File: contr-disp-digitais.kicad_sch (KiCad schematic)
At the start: 25 parts, among them U1 TL081, U2 TL081, U3 TL081

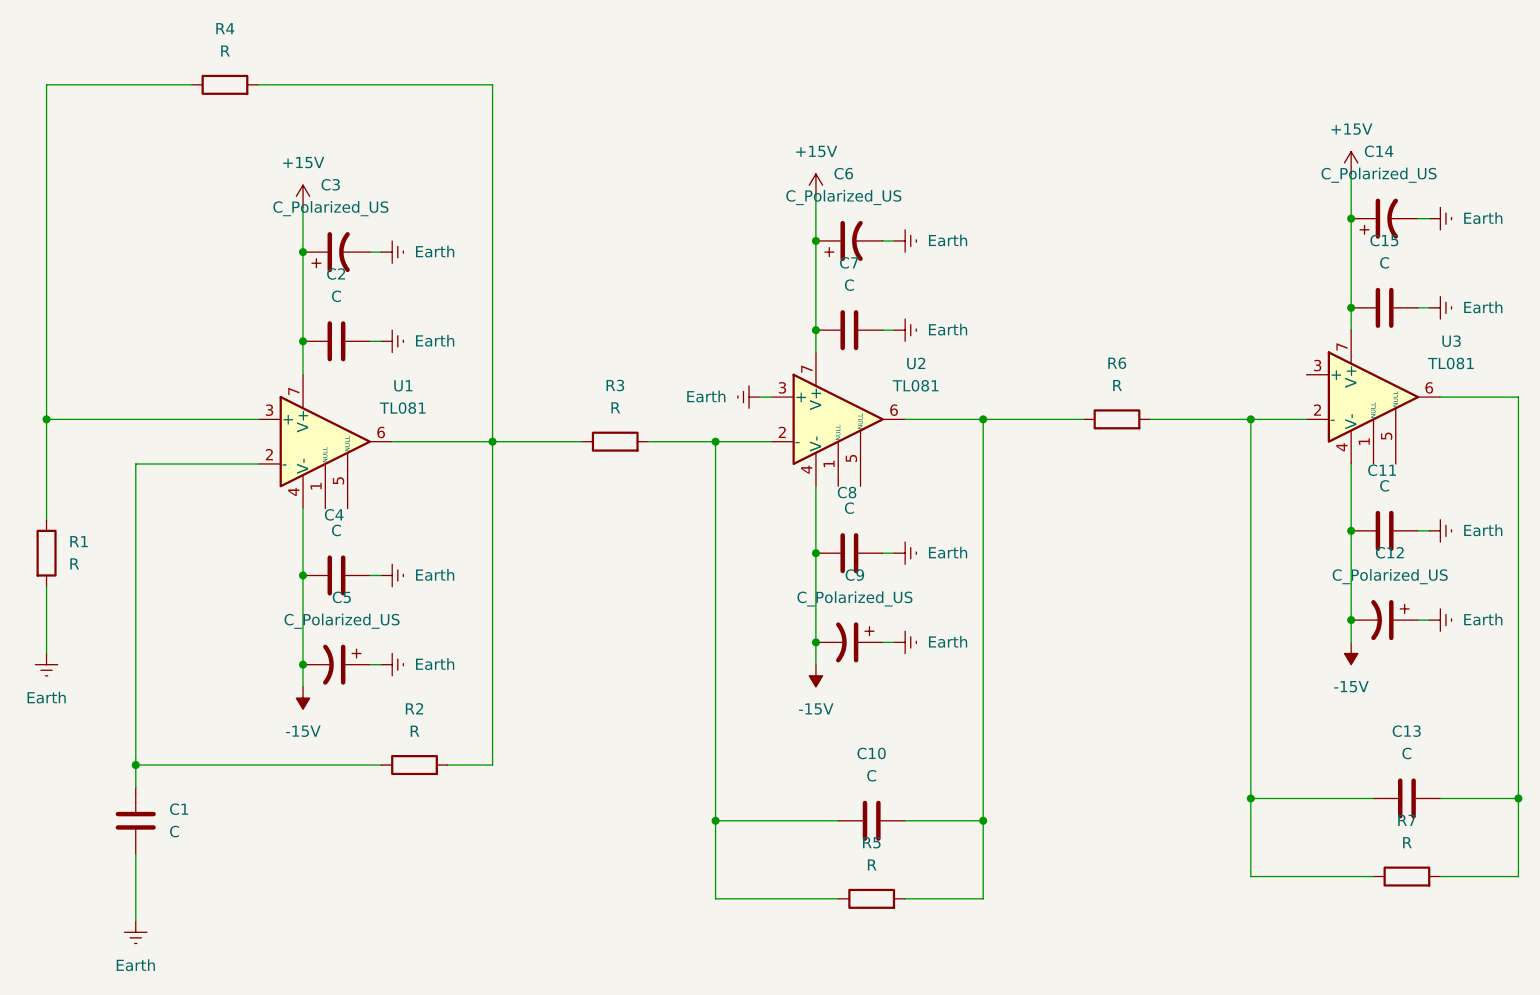
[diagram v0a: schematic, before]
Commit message: Reorganização dos esquemáticos em pages.
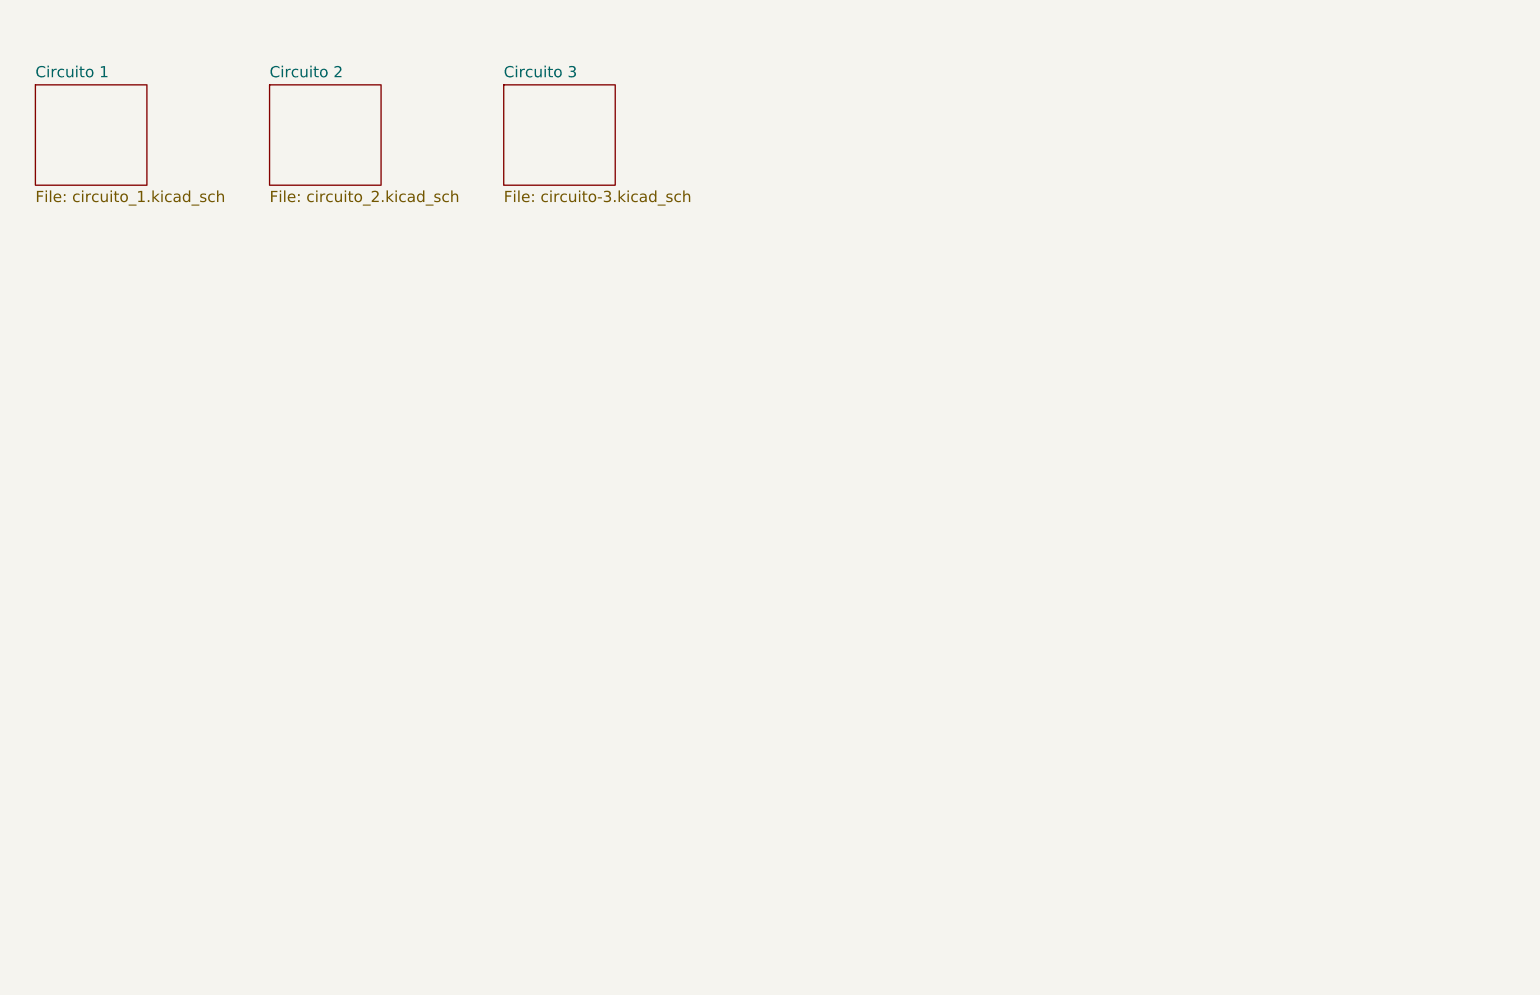
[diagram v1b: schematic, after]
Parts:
- removed C1, C10, C11, C13, C15, C2, C4, C7, C8: C, symbol Device:C
- removed C12, C14, C3, C5, C6, C9: C_Polarized_US, symbol Device:C_Polarized_US
- removed R1, R2, R3, R4, R5, R6, R7: R, symbol Device:R
- removed U1, U2, U3: TL081, symbol Amplifier_Operational:TL081
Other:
- added sheet Circuito 1 (circuito_1.kicad_sch)
- added sheet Circuito 2 (circuito_2.kicad_sch)
- added sheet Circuito 3 (circuito-3.kicad_sch)
